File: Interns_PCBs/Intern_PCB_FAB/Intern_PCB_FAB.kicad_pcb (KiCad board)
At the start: 2 copper layers, 160 x 100 mm, 104 parts, among them IC1 AND GATES, IC2 NAND (Used as AND), IC3 NAND (Used as Inverter), IC4 OR, IC5 MAX9928FAUA+, J1 AVR-ISP-6, J1 Fan, J2 Arduino Serial, J2 Coil, J3 Pi Header, J4 Conn_01x04, J5 DRIVE_GND, J7 DRIVE_5V_IN, Q1 BC557, Q2 BC547, SW1 SW_Push, U10 ATtiny85-20S

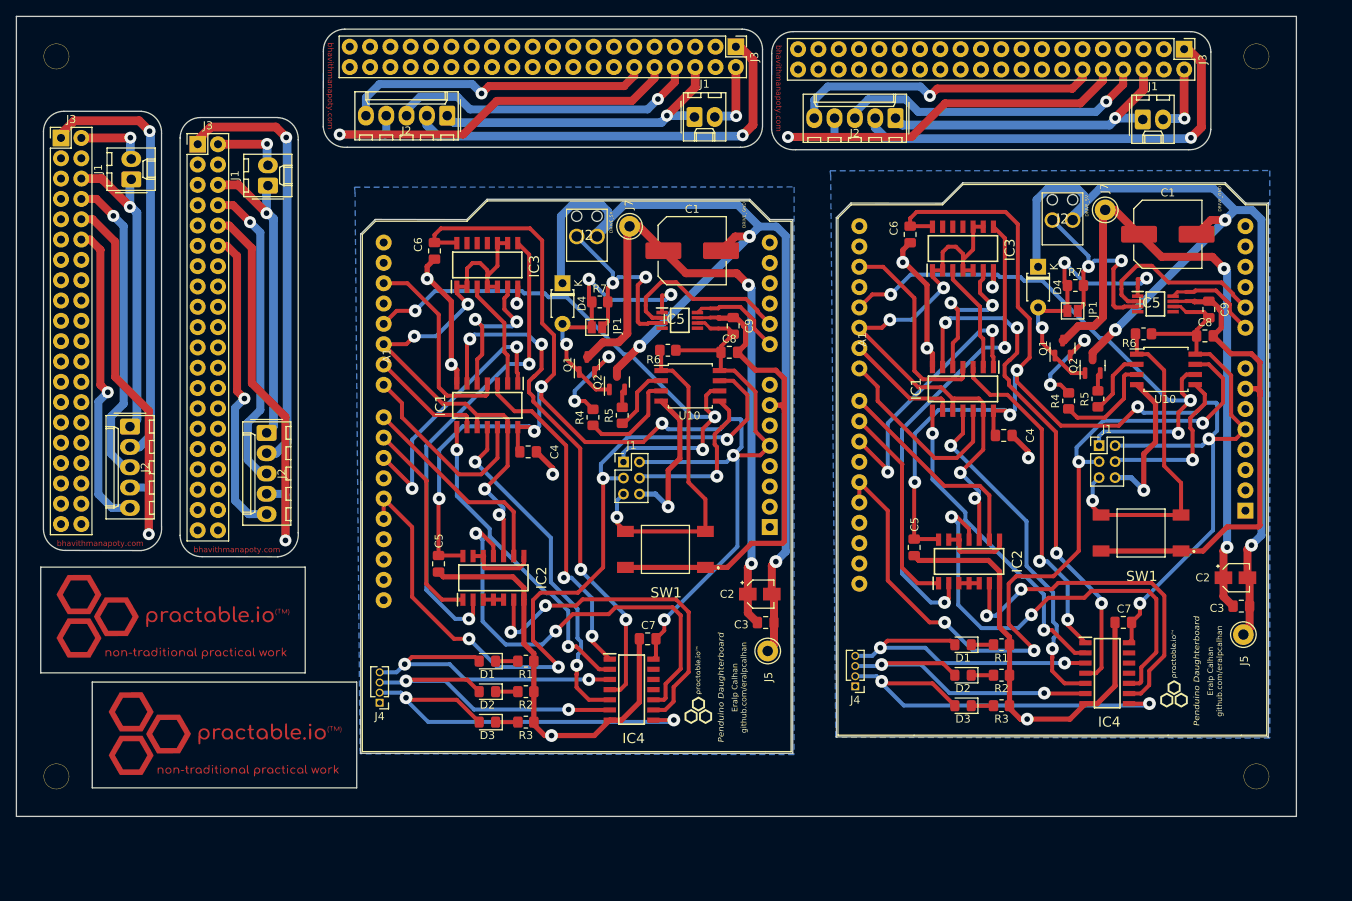
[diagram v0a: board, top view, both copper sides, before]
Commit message: 01/07 UPDATES
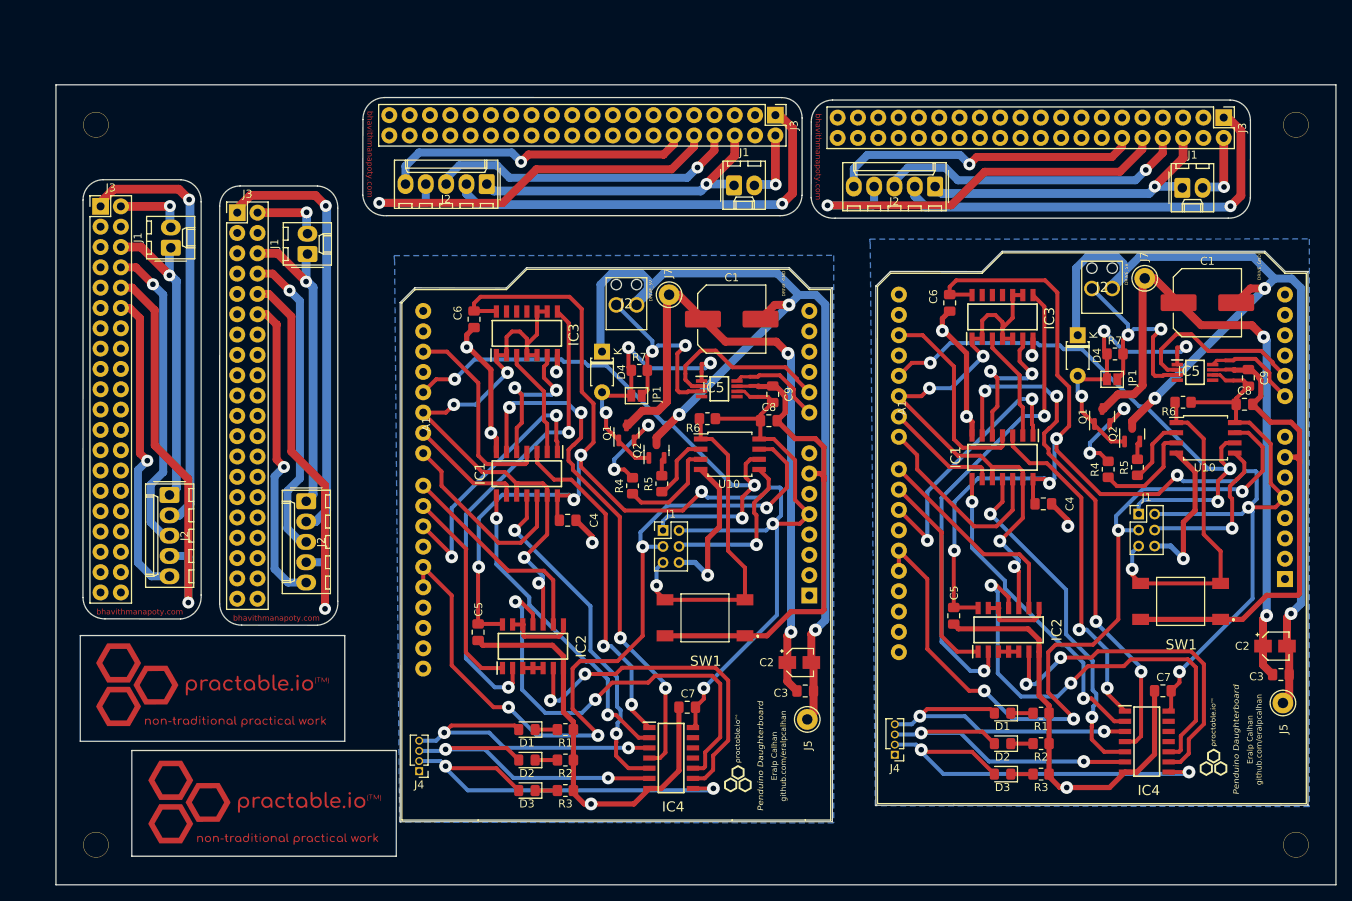
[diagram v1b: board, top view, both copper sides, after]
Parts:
- moved A1 9.88 mm to (149.8, 133.0)
- moved C9 9.88 mm to (164.9, 88.1)
- moved IC5 9.88 mm to (158.2, 87.4)
- moved J2 9.88 mm to (147.9, 77.0)
- moved NT2 9.88 mm to (222.0, 85.0)
- moved NT3 9.88 mm to (154.0, 85.1)
- moved NT6 9.88 mm to (222.0, 83.9)
- moved Q2 9.88 mm to (209.8, 93.1)
- moved R2 9.88 mm to (198.5, 131.8)
- moved R7 9.88 mm to (207.7, 83.1)
- moved G*** 9.88 mm to (94.8, 124.5)
- moved J1 9.88 mm to (106.8, 70.6)
- moved IC4 9.88 mm to (211.7, 131.6)
- moved J5 9.88 mm to (228.7, 126.7)
- moved NT4 9.88 mm to (213.2, 85.8)
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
